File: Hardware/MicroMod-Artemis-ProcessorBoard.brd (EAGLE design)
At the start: 22 x 22 mm, 40 parts, among them J1 MICROMOD-2222, U1 ARTEMIS_MODULESMD, U2 TSV524, U6 CH340E_MSOP10, Y1 32.768kHz

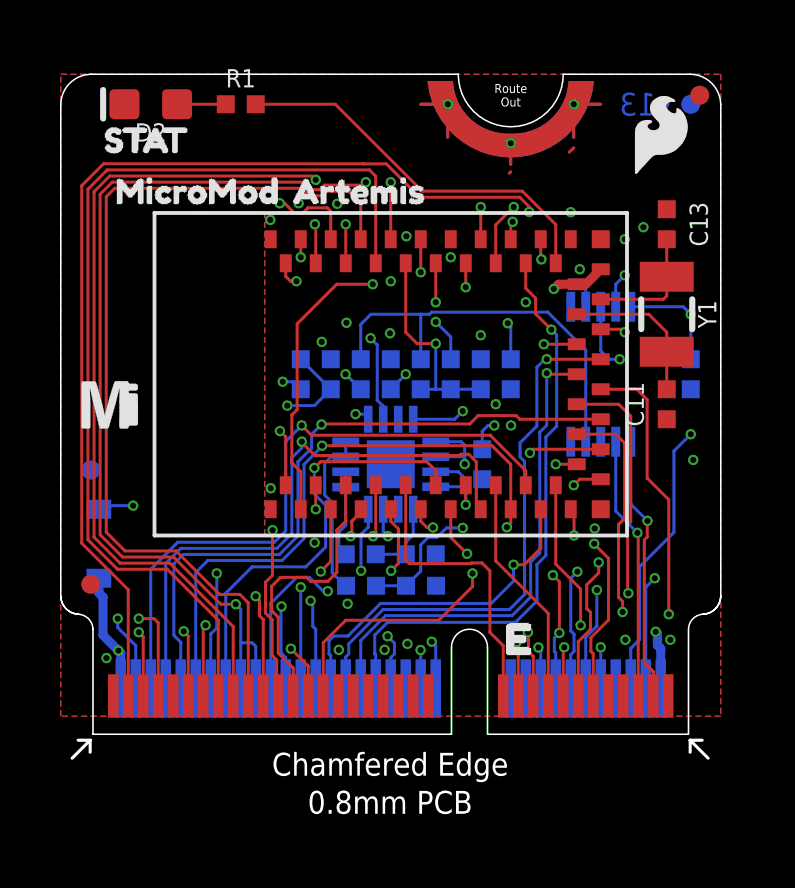
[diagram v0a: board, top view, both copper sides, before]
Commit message: Roll version to v1.4
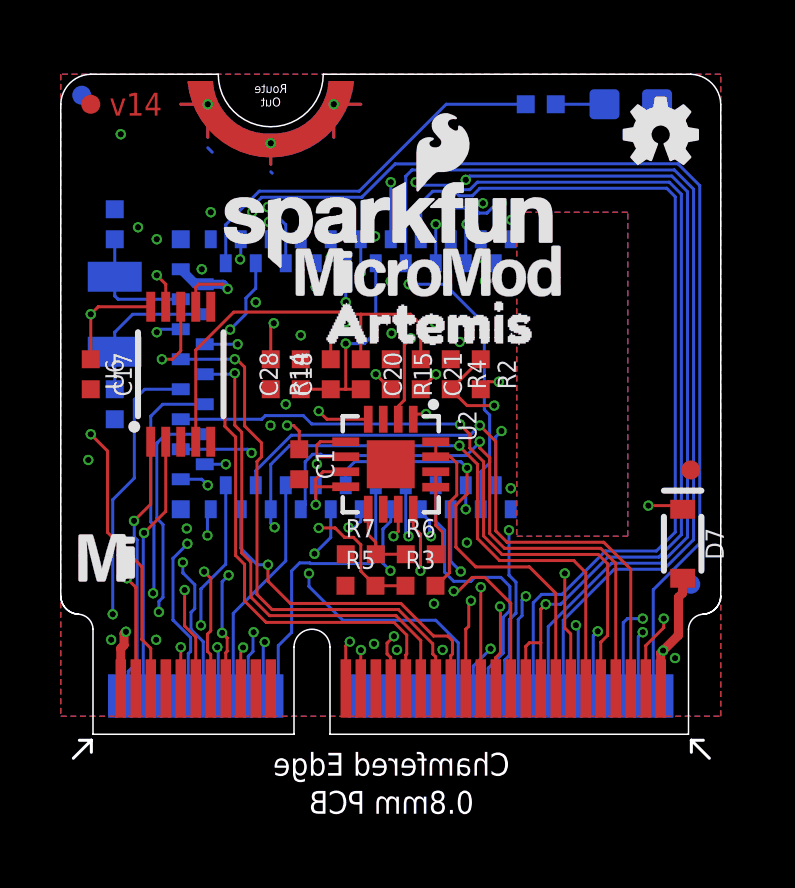
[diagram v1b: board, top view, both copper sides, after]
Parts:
- moved FRAME1 39.8 mm to (30.9, -8.89), flipped to the bottom
- moved LOGO4 27.1 mm to (-2.54, 50.8), flipped to the bottom
- moved FD2 20.6 mm to (0.70, 21.3), flipped to the bottom
- moved U$4 20.6 mm to (21.3, 19.8), flipped to the bottom
- moved C17 20.0 mm to (1.00, 12.0), flipped to the top
- moved FD1 20.0 mm to (21.0, 5.00), flipped to the bottom
- moved FD3 20.0 mm to (1.00, 21.0), flipped to the top
- moved FD4 20.0 mm to (21.0, 8.81), flipped to the top
- moved U$3 19.8 mm to (20.9, 18.1), flipped to the bottom
- moved D7 19.5 mm to (20.7, 6.35), flipped to the top
- moved U$7 19.0 mm to (1.50, 5.90), flipped to the top
- moved U$1 18.8 mm to (20.4, 11.0), flipped to the bottom
- moved C11 18.4 mm to (1.80, 11.0), flipped to the bottom
- moved C13 18.4 mm to (1.80, 17.0), flipped to the bottom
- moved Y1 18.4 mm to (1.80, 14.0), flipped to the bottom
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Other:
- outline, holes or cut-outs redrawn
- board text added: "v14"
- board text removed: "v13"
